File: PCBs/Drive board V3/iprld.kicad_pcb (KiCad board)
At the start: 2 copper layers, 100 x 80.1 mm, 44 parts, among them IC4 ADS1115IDGSR, J2 Conn_01x04_Pin, U15 AMS1117-3.3, U9 TCA9548APWR

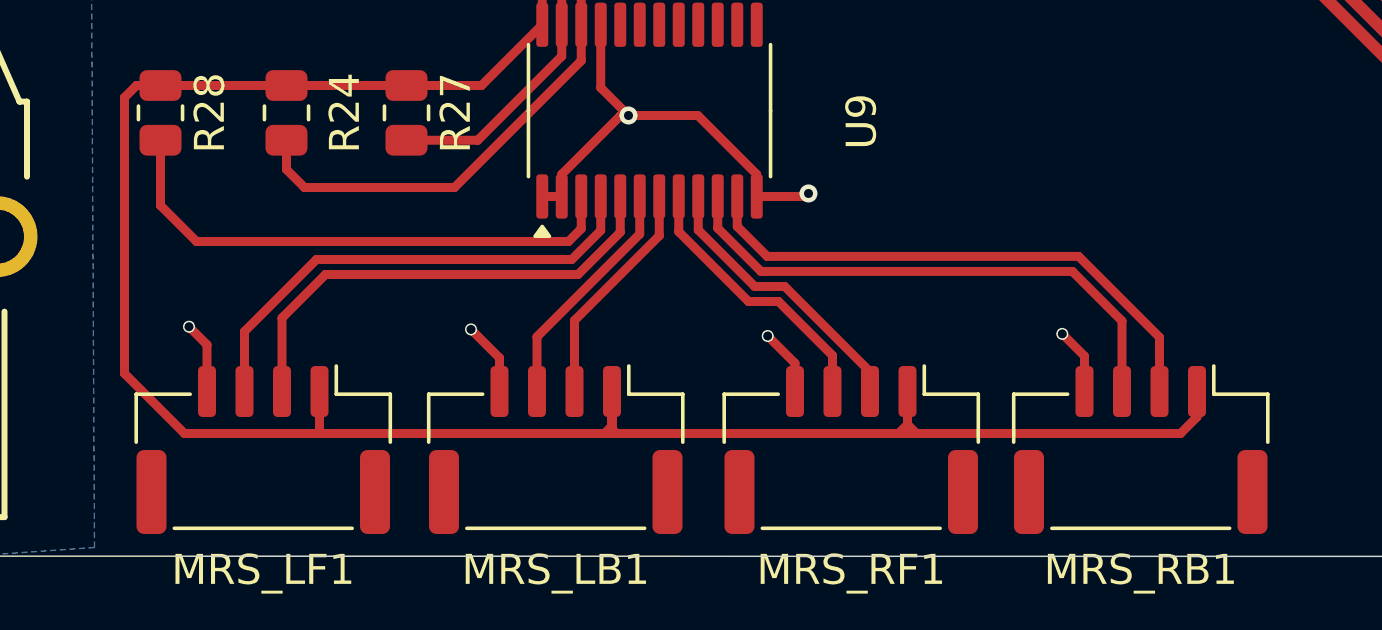
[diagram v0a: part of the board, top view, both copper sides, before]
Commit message: i2c breakout correction, fuck you Maciej
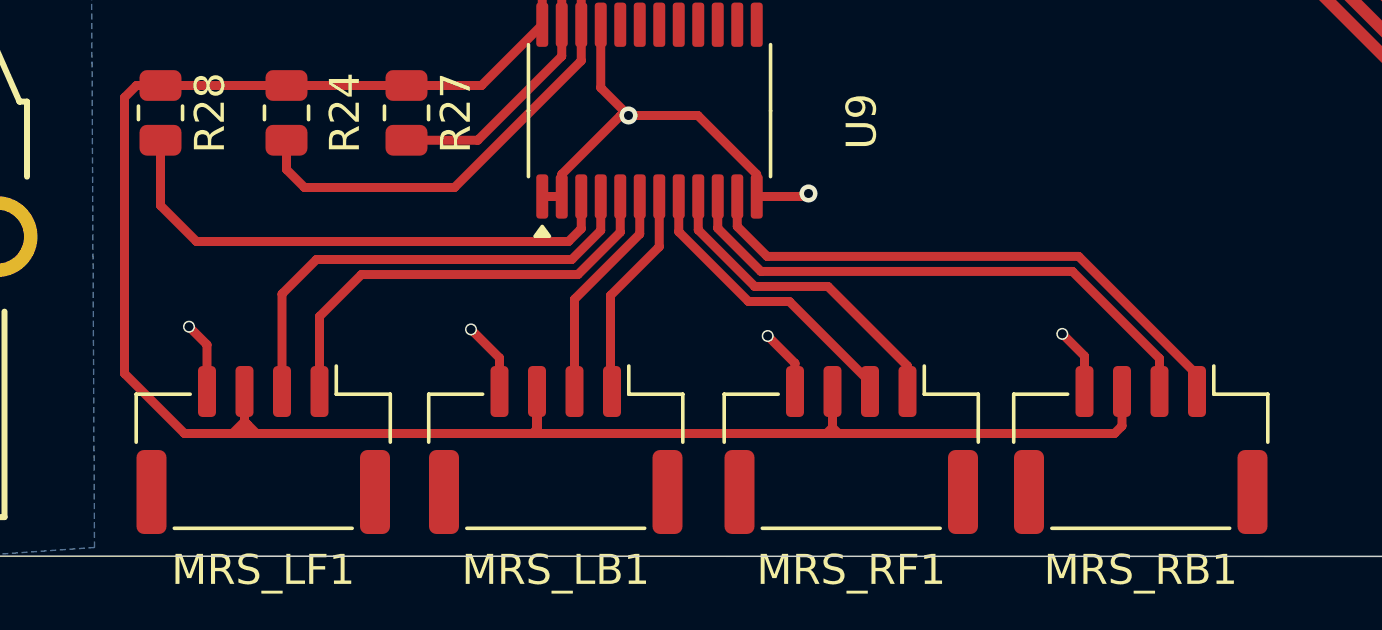
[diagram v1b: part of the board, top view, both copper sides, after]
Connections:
- MRS_LB1 pad 1: +3.3V -> /SCL_LB
- MRS_LB1 pad 2: /SCL_LB -> /SDA_LB
- MRS_LB1 pad 3: /SDA_LB -> +3.3V
- MRS_LF1 pad 1: +3.3V -> /SCL_LF
- MRS_LF1 pad 2: /SCL_LF -> /SDA_LF
- MRS_LF1 pad 3: /SDA_LF -> +3.3V
- MRS_RB1 pad 1: +3.3V -> /SCL_RB
- MRS_RB1 pad 2: /SCL_RB -> /SDA_RB
- MRS_RB1 pad 3: /SDA_RB -> +3.3V
- MRS_RF1 pad 1: +3.3V -> /SCL_RF
- MRS_RF1 pad 2: /SCL_RF -> /SDA_RF
- MRS_RF1 pad 3: /SDA_RF -> +3.3V
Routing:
- net +3.3V: track 190.6 -> 188.9 mm
- net /SDA_RF: track 9.21 -> 10.6 mm
- net /SCL_RF: track 9.46 -> 10.8 mm
- net /SCL_LF: track 16.1 -> 14.9 mm
- net /SDA_LB: track 7.92 -> 7.40 mm
- net /SDA_RB: track 18.2 -> 18.7 mm
- net /SDA_LF: track 16.4 -> 15.9 mm
- net /SCL_RB: track 18.4 -> 18.9 mm
